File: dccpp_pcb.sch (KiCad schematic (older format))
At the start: 60 parts, among them J1 USB_B_Micro, J10 OSTTC022162, J11 OSTTC022162, J12 OSTTC022162, J2 AVR-ISP-6, J3 OSTTC022162, J4 OSTTC022162, J5 OSTTC022162, J6 OSTTC022162, J7 OSTTC022162, J8 OSTTC022162, J9 OSTTC022162, U1 ATmega32U4-AU, U2 74HC04, U3 IFX007T, U4 IFX007T, U5 IFX007T, U6 IFX007T, Y1 16MHz

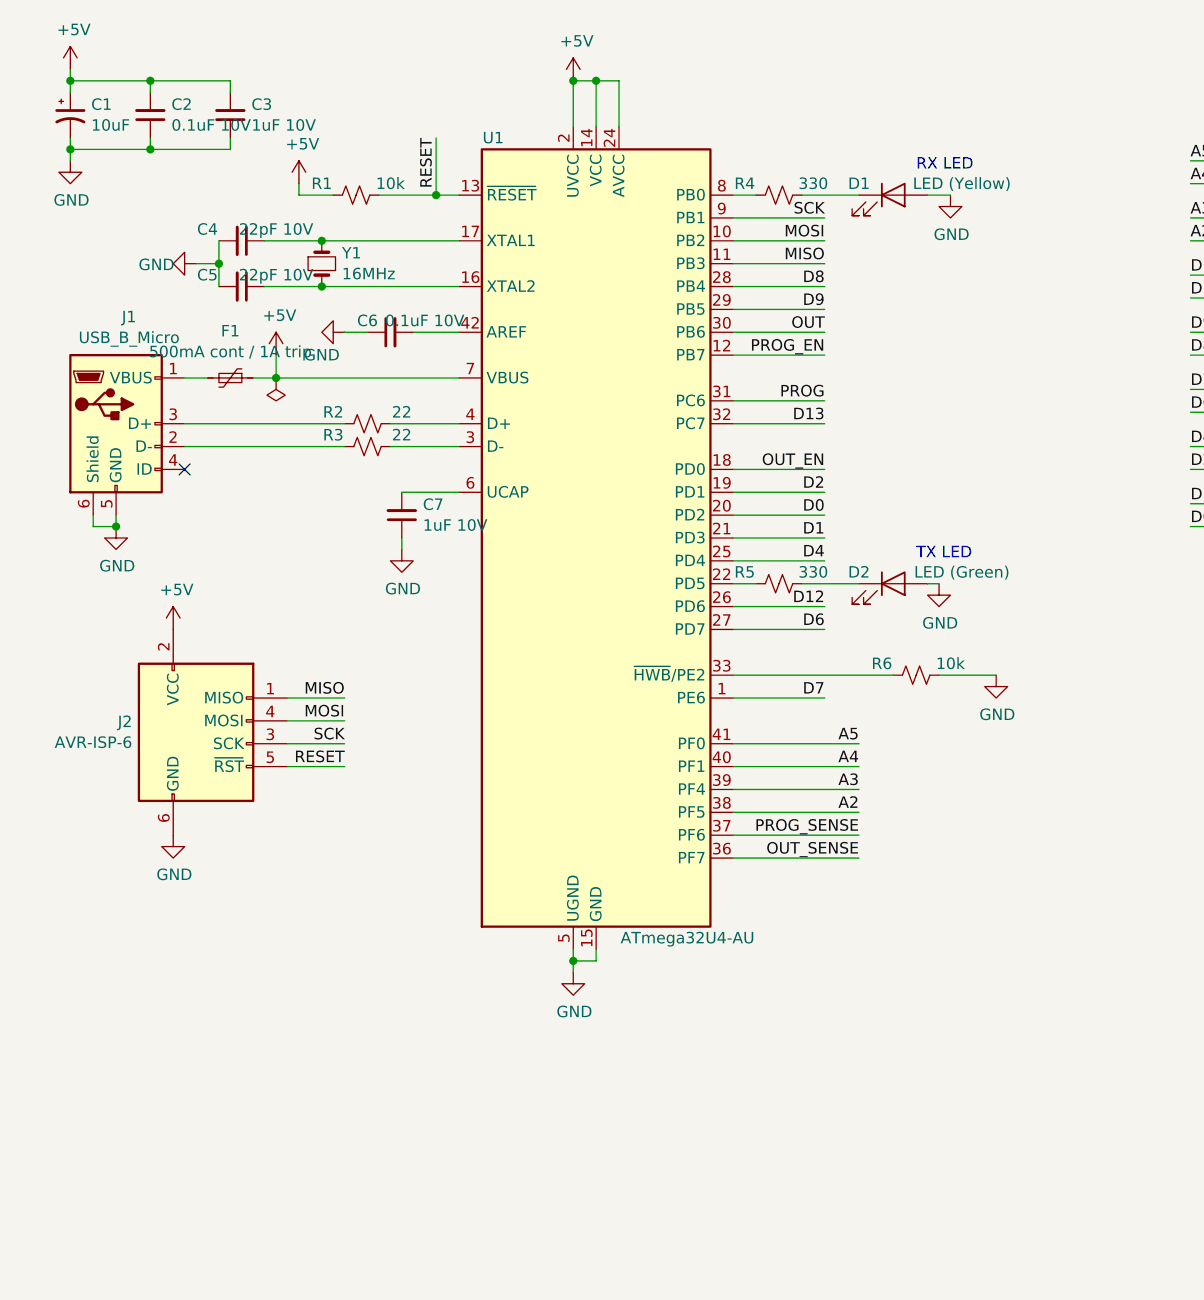
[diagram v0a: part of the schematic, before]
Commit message: More routing
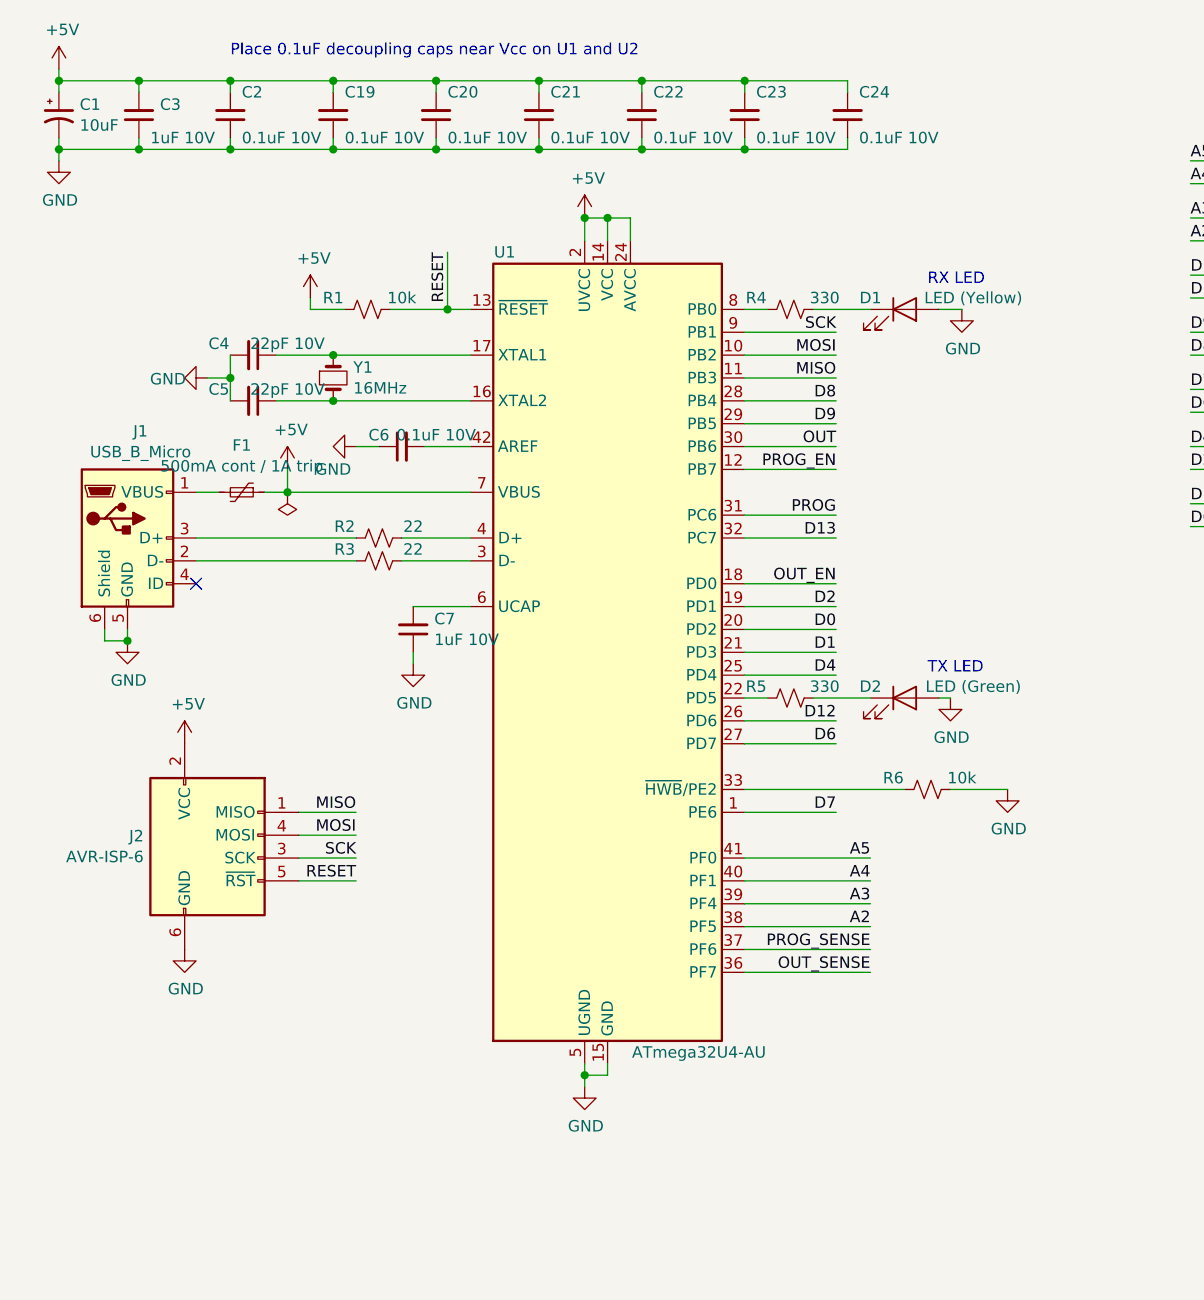
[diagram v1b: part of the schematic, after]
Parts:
- added C19, C20, C21, C22, C23, C24: 0.1uF 10V, Capacitor_SMD:C_0603_1608Metric_Pad1.05x0.95mm_HandSolder, symbol Device:C_Small
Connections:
- net +5V: now also C19.2, C20.2, C21.2, C22.2, C23.2, C24.2
- net GND: now also C19.1, C20.1, C21.1, C22.1, C23.1, C24.1
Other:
- note added: "Place 0.1uF decoupling caps near Vcc on U1 and U2"
- moved on the sheet: C1, C2, C3, C4, C5, C6, C7, D1, D2, F1, J1, J2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
